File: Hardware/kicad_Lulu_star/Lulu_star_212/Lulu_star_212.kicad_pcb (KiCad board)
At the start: 2 copper layers, 16.7 x 14.9 mm, 7 parts, among them J1 Conn_01x03_Female, J1 Soldering_pad, Q1 Q_NMOS_GSD, T1 Q_NPN_BEC

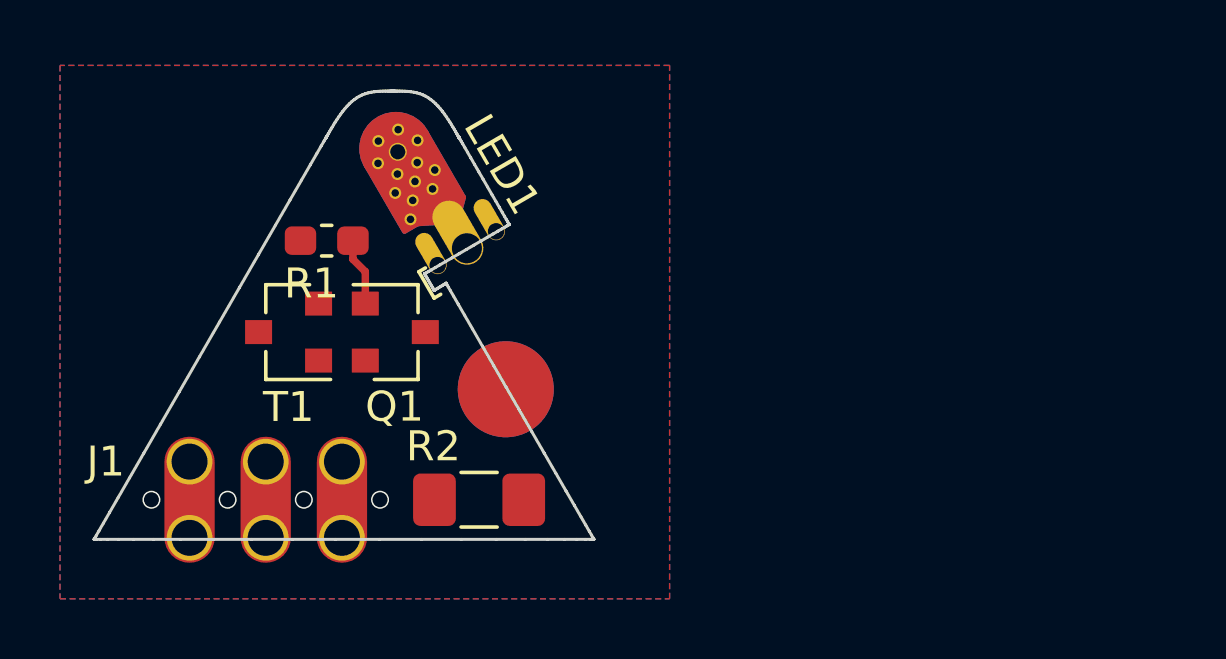
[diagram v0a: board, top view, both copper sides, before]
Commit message: PCB in progress
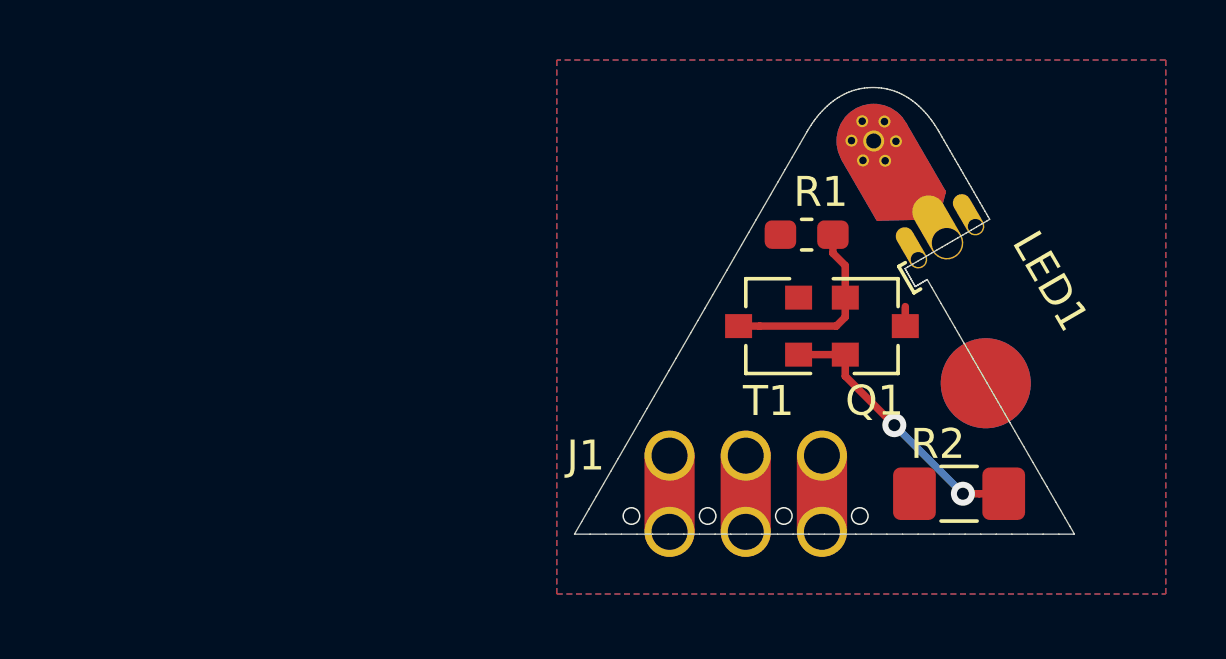
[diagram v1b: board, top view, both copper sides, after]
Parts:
- moved J1 16.0 mm to (139.7, 108.3)
- moved T1 16.0 mm to (140.5, 102.7)
- moved J1 16.0 mm to (147.7, 104.6)
- moved Q1 16.0 mm to (144.0, 102.7)
- moved R2 16.0 mm to (146.8, 108.3)
- moved R1 16.0 mm to (141.7, 99.6)
- moved LED1 16.0 mm to (146.4, 99.9)
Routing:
- net Net-(Q1-Pad2): track 0.00 -> 9.05 mm, vias 0 -> 2
- net Net-(Q1-Pad1): track 2.27 -> 6.60 mm
- net +3V3: track 0.00 -> 1.27 mm
- net Net-(LED1-Pad1): track 0.00 -> 0.65 mm
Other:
- outline, holes or cut-outs redrawn
